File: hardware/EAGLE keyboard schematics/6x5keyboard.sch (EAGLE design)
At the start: 70 parts

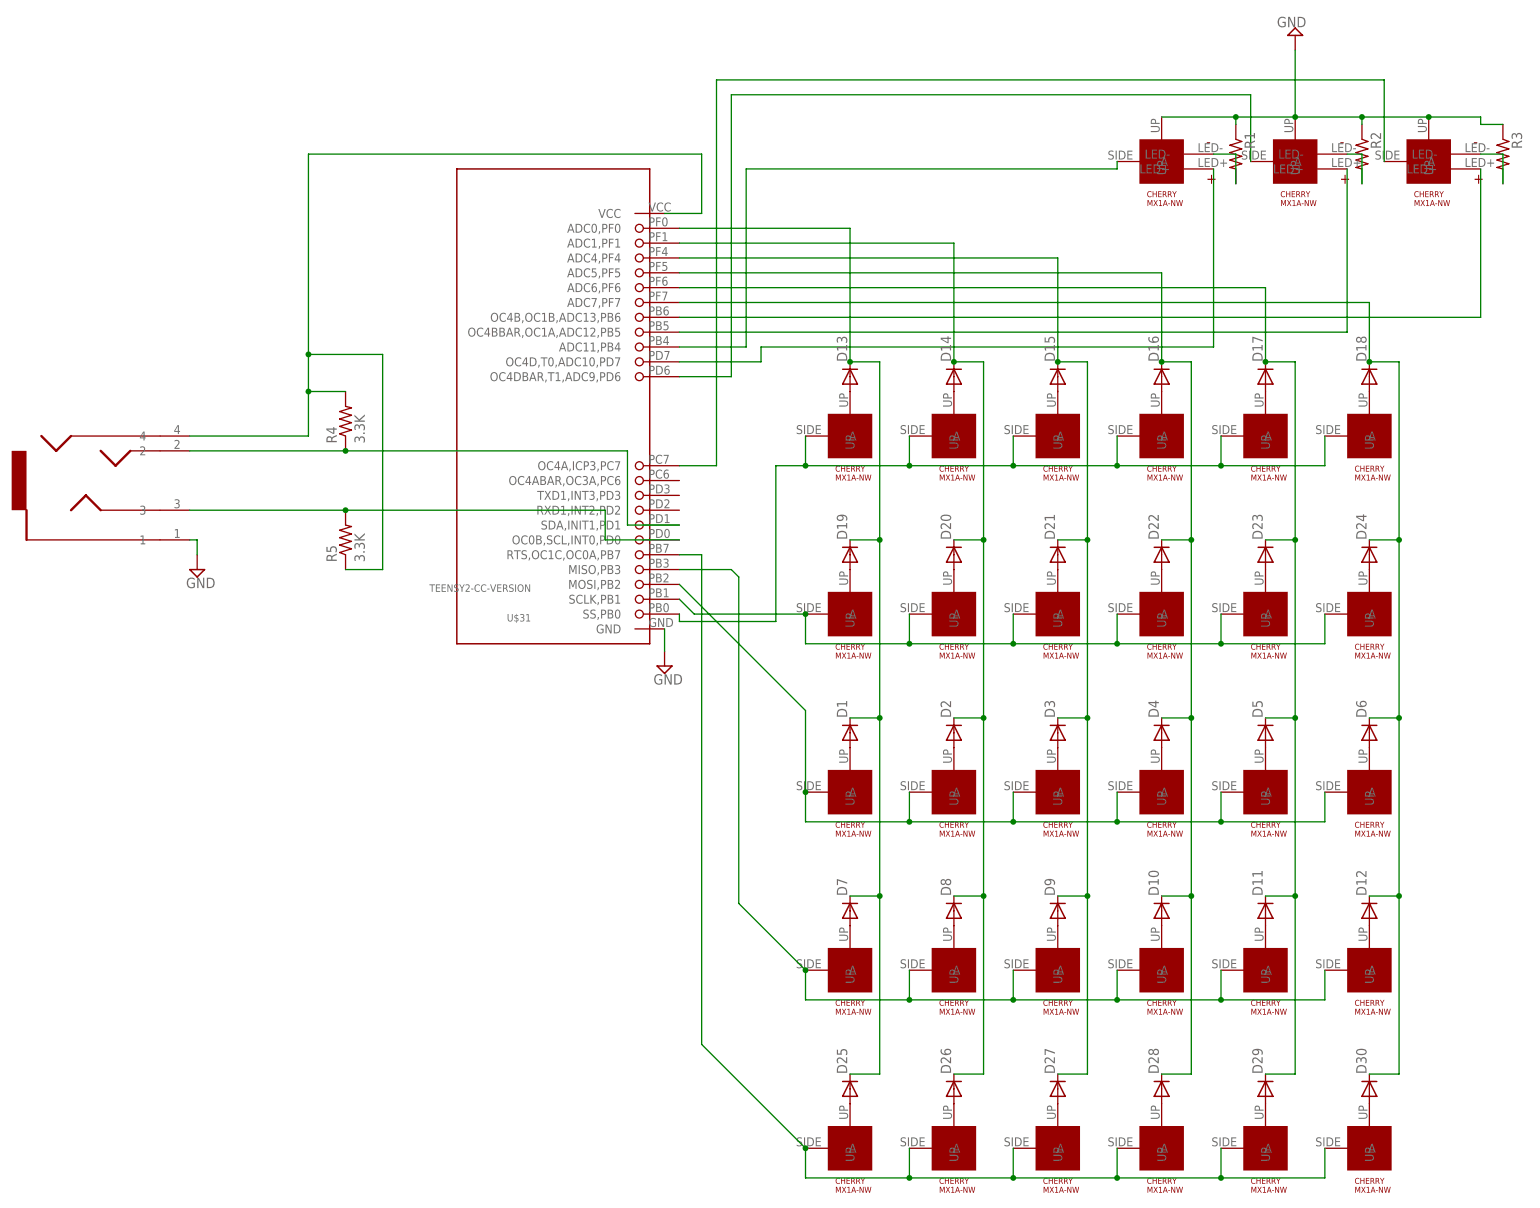
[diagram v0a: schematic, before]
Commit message: work
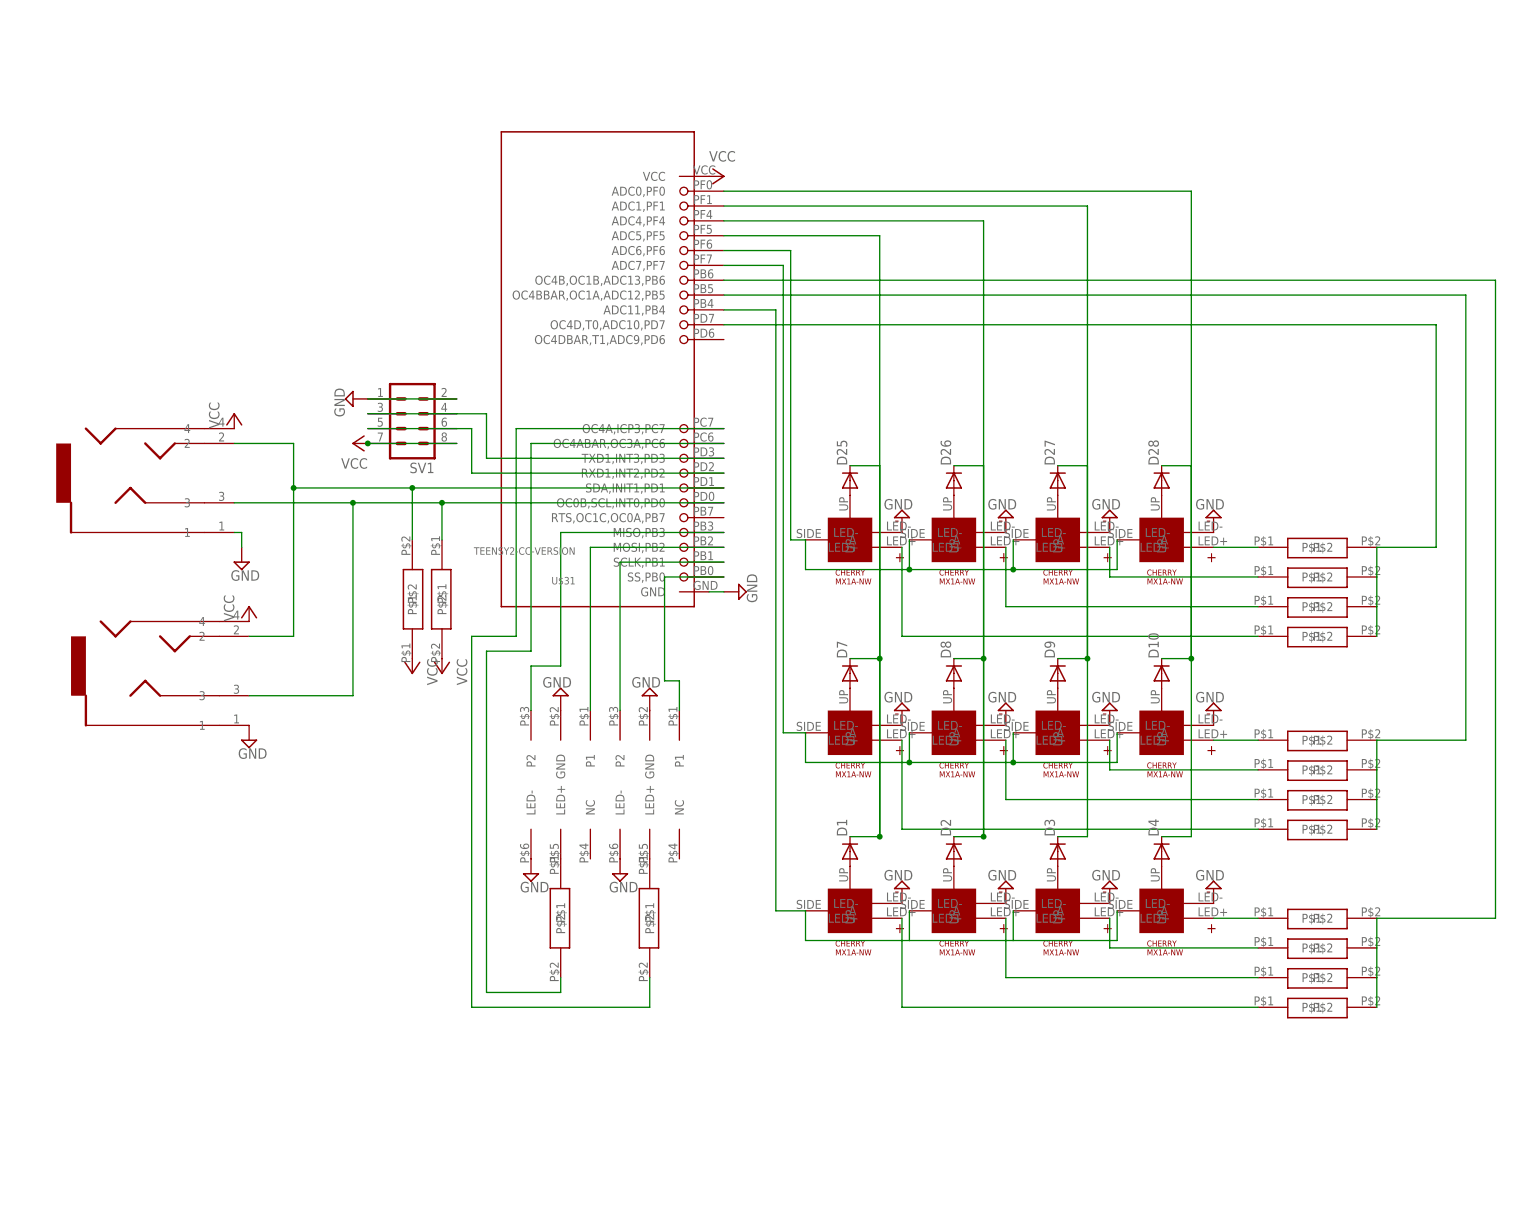
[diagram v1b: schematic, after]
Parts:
- removed D11, D12, D13, D14, D15, D16, D17, D18, D19, D20, D21, D22, D23, D24, D29, D30, D5, D6: 1N4148DO35-7, diode:1N4148DO35-7
- removed R1, R2, R3: (no value), rcl:R-US_0207/10
- removed R4, R5: 3.3K, resistor:R-US_0207/10
- removed U$32, U$33, U$34: CHERRY-MX1A-E1NW-LED, my_parts:CHERRY-MX1A-E1NW-LED
- added COMM1: SJ-43514_HEADPHONES_3.5MM_X4, my_parts:SJ-43514_HEADPHONES_3.5MM_X4
- added SV1: (no value), con-lstb:MA04-2
- U$1, U$10, U$2, U$25, U$26, U$27, U$28, U$3, U$4, U$7, U$8, U$9: value CHERRY-MX1A-E1NW -> CHERRY-MX1A-E1NW-LED; device my_parts:CHERRY-MX1A-E1NW -> my_parts:CHERRY-MX1A-E1NW-LED
- U$11, U$12, U$13, U$14, U$15, U$16, U$17, U$18, U$19, U$20, U$21, U$22, U$29, U$30, U$5, U$6: value CHERRY-MX1A-E1NW -> RESISTORBIGPAD; device my_parts:CHERRY-MX1A-E1NW -> my_parts:RESISTORBIGPAD
- U$23, U$24: value CHERRY-MX1A-E1NW -> NKK_GW_SERIES; device my_parts:CHERRY-MX1A-E1NW -> my_parts:NKK_GW_SERIES
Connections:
- removed net N$43: R2.2, U$33.LED-
- removed net N$44: R3.2, U$34.LED-
- removed net N$46: U$31.OC4BBAR,OC1A,ADC12,PB5, U$33.LED+
- removed net N$47: U$31.OC4B,OC1B,ADC13,PB6, U$34.LED+
- removed net N$48: U$31.ADC11,PB4, U$32.A
- removed net N$53: COMM.2, R4.1, U$31.SDA,INIT1,PD1
- removed net N$54: U$31.OC4D,T0,ADC10,PD7, U$32.LED+
- new net VCC: COMM.4, COMM1.4, SV1.7, SV1.8, U$21.P$1, U$22.P$2, U$31.VCC
- net GND: now also COMM1.1, SV1.1, SV1.2, U$1.LED-, U$10.LED-, U$2.LED-, U$23.GND, U$23.LED-, U$24.GND, U$24.LED-, U$25.LED-, U$26.LED-, U$27.LED-, U$28.LED-, U$3.LED-, U$4.LED-, U$7.LED-, U$8.LED-, U$9.LED-; no longer R1.1, R2.1, R3.1, U$32.UP, U$33.UP, U$34.UP
- net N$11: now also U$11.P$1, U$3.LED+; no longer D11.A, U$11.UP
- net N$12: now also U$1.LED+, U$6.P$1; no longer D12.A, U$12.UP
- net N$13: now also U$2.LED+, U$5.P$1; no longer D13.A, U$13.UP
- net N$14: now also U$30.P$2, U$31.OC4A,ICP3,PC7; no longer D14.A, U$14.UP
- net N$15: now also U$24.LED+, U$30.P$1; no longer D15.A, U$15.UP
- net N$16: now also COMM.2, COMM1.2, U$21.P$2, U$31.SDA,INIT1,PD1; no longer D16.A, U$16.UP
- net N$17: now also U$29.P$2, U$31.OC4ABAR,OC3A,PC6; no longer D17.A, U$17.UP
- net N$18: now also U$10.LED+, U$13.P$1; no longer D18.A, U$18.UP
- net N$19: now also U$14.P$1, U$9.LED+; no longer D19.A, U$19.UP
- net N$20: now also U$15.P$1, U$8.LED+; no longer D20.A, U$20.UP
- net N$21: now also U$16.P$1, U$7.LED+; no longer D21.A, U$21.UP
- net N$22: now also U$24.P1, U$31.SS,PB0; no longer D22.A, U$22.UP
- net N$23: now also U$17.P$1, U$28.LED+; no longer D23.A, U$23.UP
- net N$24: now also U$18.P$1, U$27.LED+; no longer D24.A, U$24.UP
- net N$29: now also U$19.P$1, U$26.LED+; no longer D29.A, U$29.UP
- net N$30: now also U$20.P$1, U$25.LED+; no longer D30.A, U$30.UP
- net N$31: now also U$31.ADC5,PF5; no longer D13.C, D19.C, U$31.ADC0,PF0
- net N$32: now also U$31.ADC4,PF4; no longer D14.C, D20.C, U$31.ADC1,PF1
- net N$33: now also U$31.ADC1,PF1; no longer D15.C, D21.C, U$31.ADC4,PF4
- net N$34: now also U$31.ADC0,PF0; no longer D16.C, D22.C, U$31.ADC5,PF5
- net N$35: now also U$24.P2, U$31.SCLK,PB1; no longer D11.C, D17.C, D23.C, D29.C, D5.C, U$31.ADC6,PF6
- net N$36: now also U$23.P1, U$31.MOSI,PB2; no longer D12.C, D18.C, D24.C, D30.C, D6.C, U$31.ADC7,PF7
- net N$37: now also SV1.3, SV1.4, U$31.TXD1,INT3,PD3; no longer U$19.A, U$20.A, U$21.A, U$22.A, U$23.A, U$24.A, U$31.SCLK,PB1
- net N$38: now also U$31.ADC11,PB4; no longer U$31.MOSI,PB2, U$5.A, U$6.A
- net N$39: now also U$31.ADC7,PF7; no longer U$11.A, U$12.A, U$31.MISO,PB3
- net N$40: now also U$31.ADC6,PF6; no longer U$29.A, U$30.A, U$31.RTS,OC1C,OC0A,PB7
- net N$41: now also SV1.5, SV1.6, U$31.RXD1,INT2,PD2; no longer U$13.A, U$14.A, U$15.A, U$16.A, U$17.A, U$18.A, U$31.SS,PB0
- net N$42: now also U$23.P2, U$31.MISO,PB3; no longer R1.2, U$32.LED-
- net N$49: now also U$11.P$2, U$12.P$2, U$31.OC4B,OC1B,ADC13,PB6, U$5.P$2, U$6.P$2; no longer U$31.OC4DBAR,T1,ADC9,PD6, U$33.A
- net N$5: now also U$12.P$1, U$4.LED+; no longer D5.A, U$5.UP
- net N$50: now also U$13.P$2, U$14.P$2, U$15.P$2, U$16.P$2, U$31.OC4BBAR,OC1A,ADC12,PB5; no longer U$31.OC4A,ICP3,PC7, U$34.A
- net N$51: now also U$17.P$2, U$18.P$2, U$19.P$2, U$20.P$2, U$31.OC4D,T0,ADC10,PD7; no longer COMM.4, R4.2, R5.1, U$31.VCC
- net N$52: now also COMM1.3, U$22.P$1; no longer R5.2
- net N$6: now also U$23.LED+, U$29.P$1; no longer D6.A, U$6.UP
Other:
- moved on the sheet: D1, D10, D2, D25, D26, D27, D28, D3, D4, D7, D8, D9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
